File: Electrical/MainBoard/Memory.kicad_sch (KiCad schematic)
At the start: 4 parts, among them J17 MEM2061-01-188-00-A, U15 M95M01-DFMN6TP

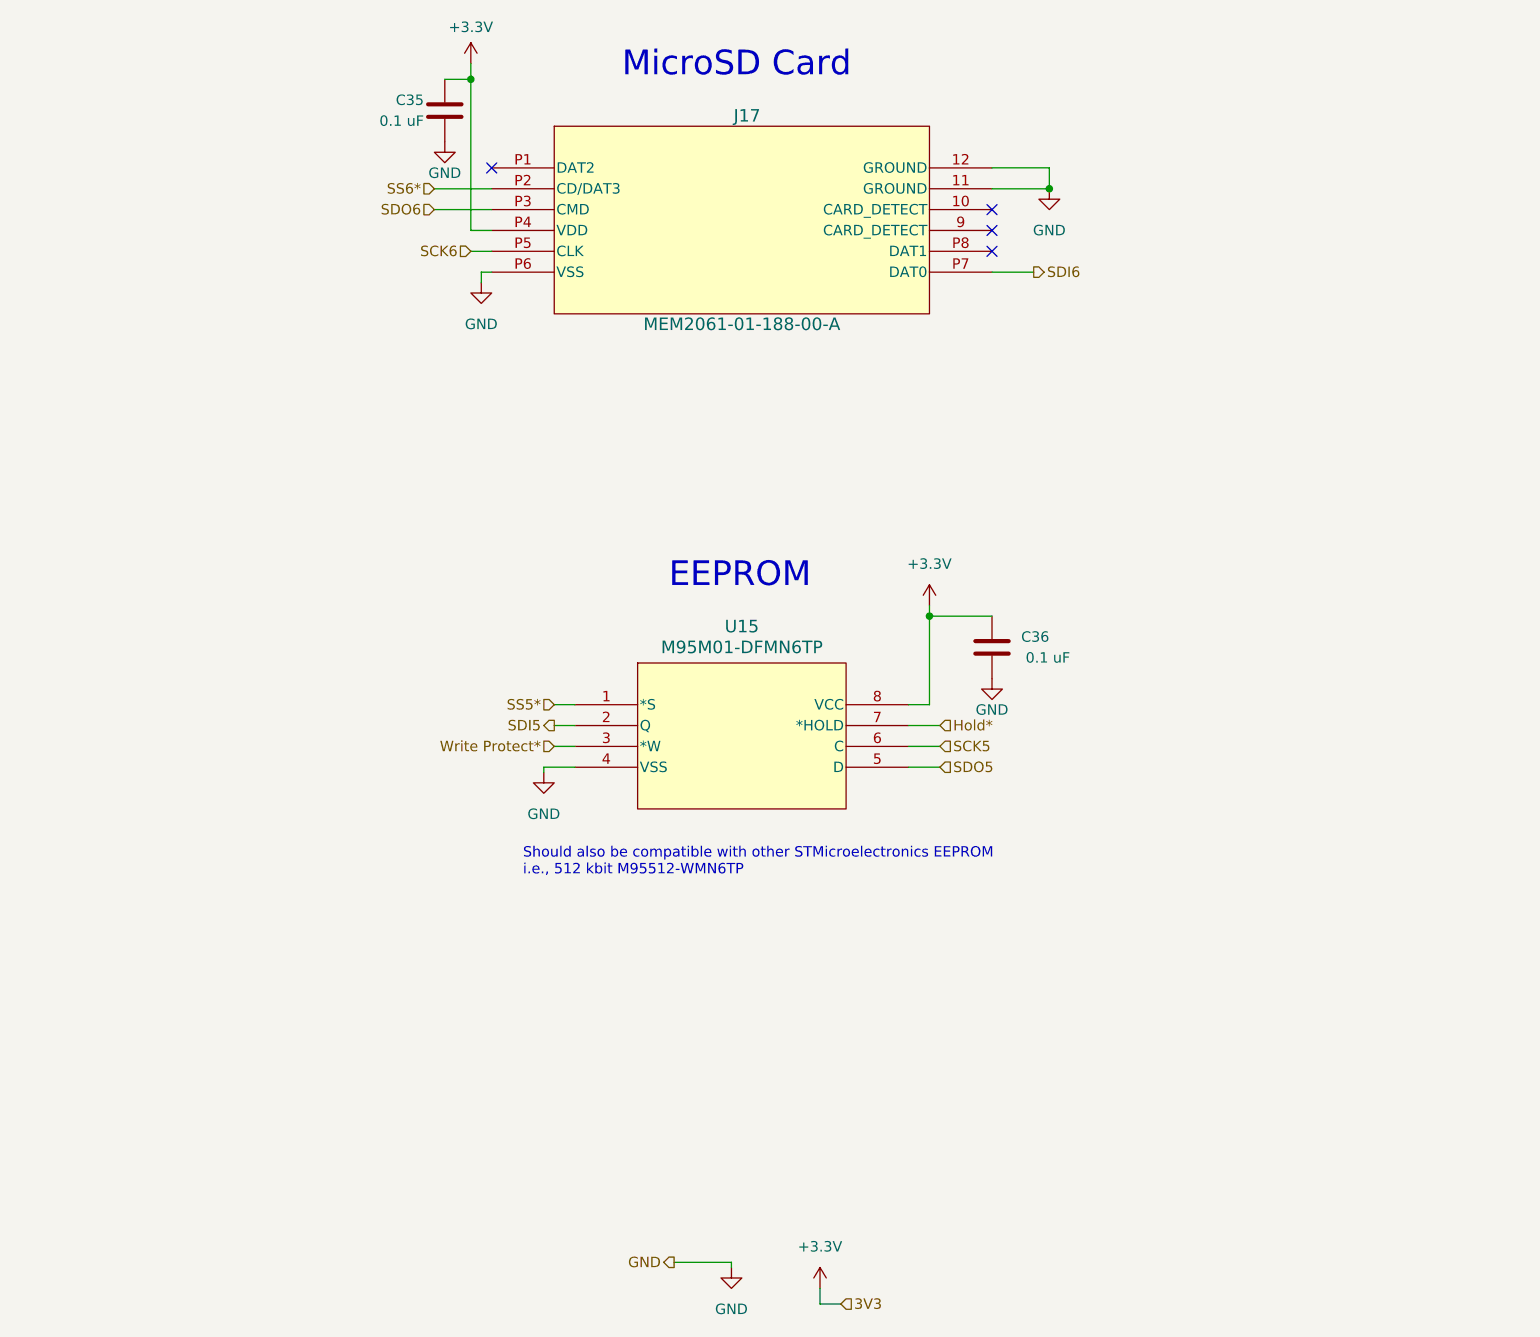
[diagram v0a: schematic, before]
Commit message: Add updated pdf schematic
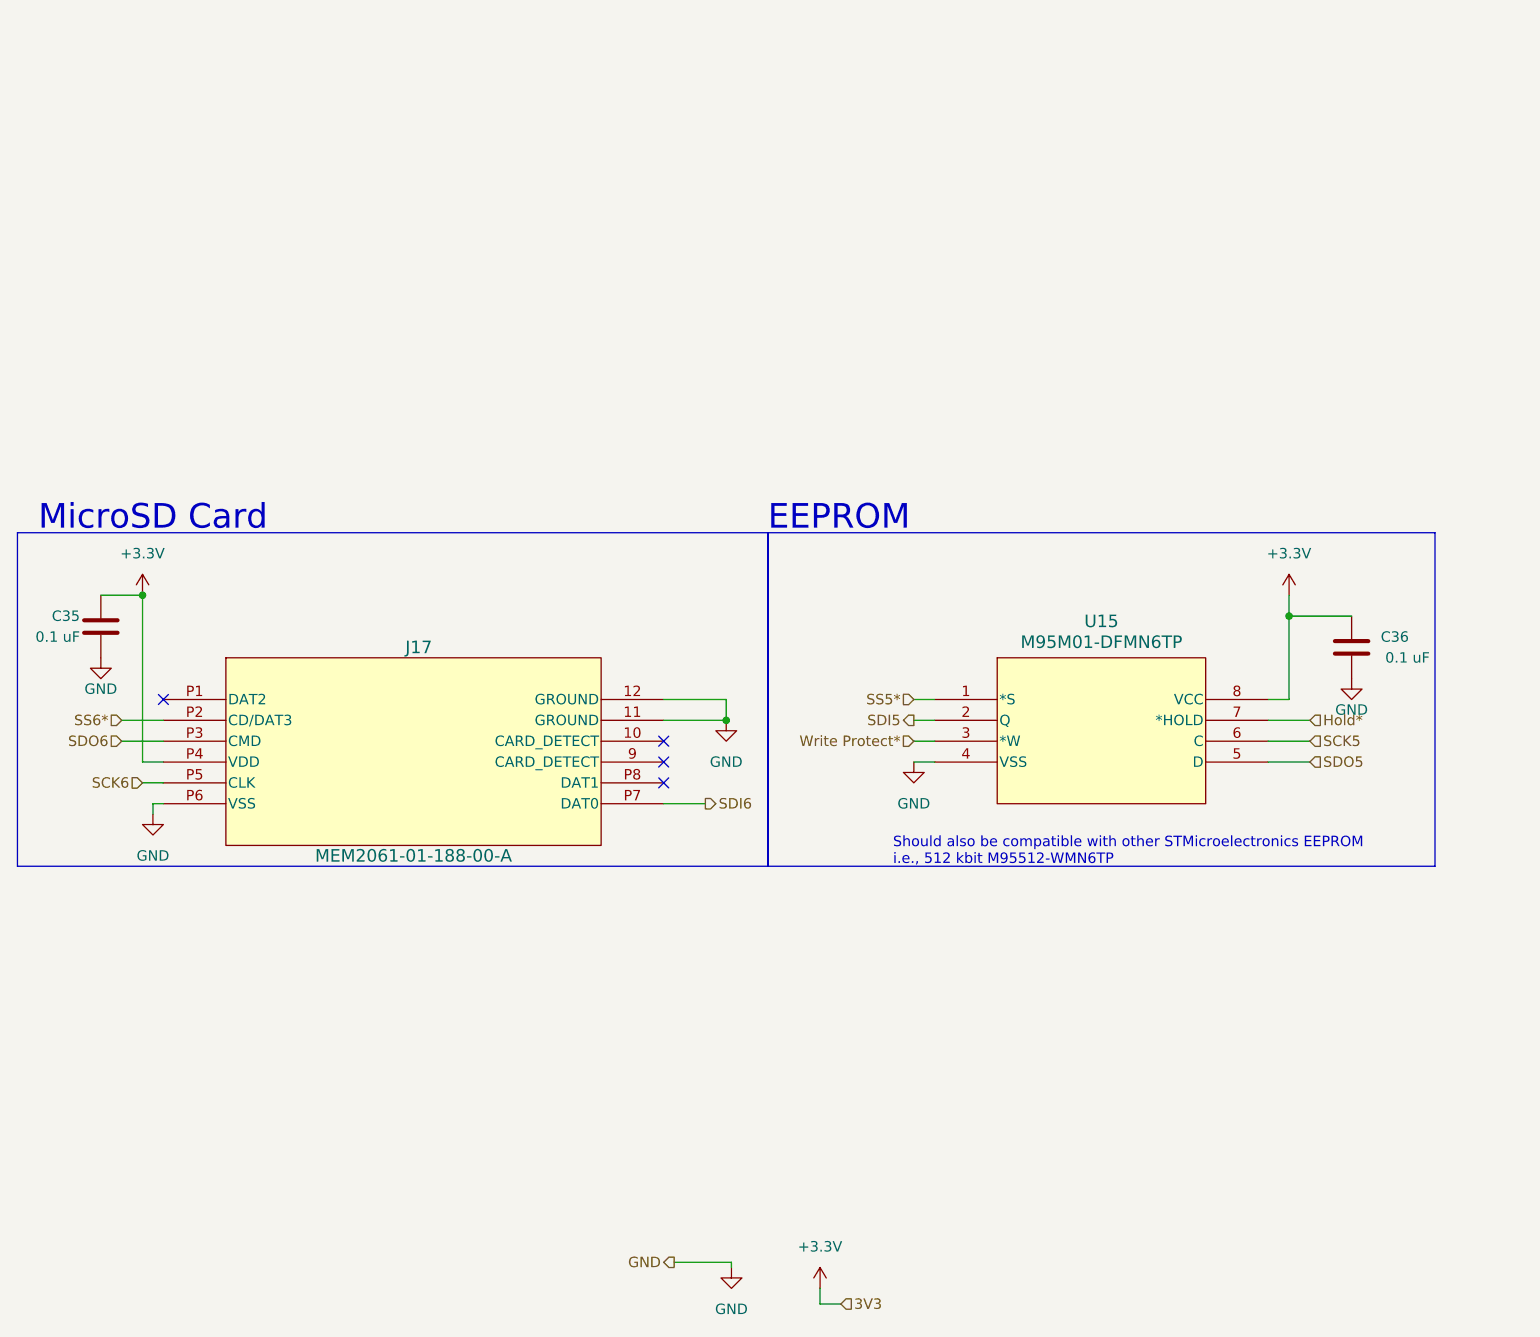
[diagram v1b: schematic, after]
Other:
- moved on the sheet: C35, C36, J17, U15
